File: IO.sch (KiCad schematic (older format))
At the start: 5 parts

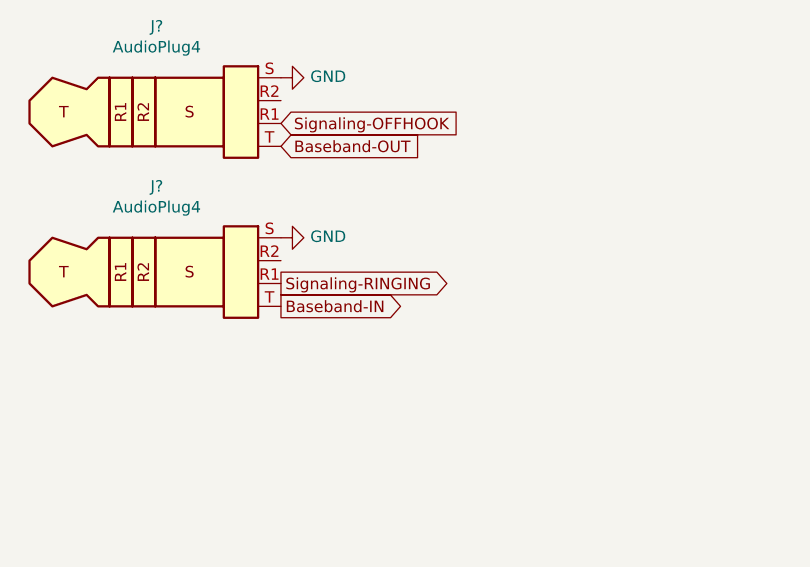
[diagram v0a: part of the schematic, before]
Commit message: more updates
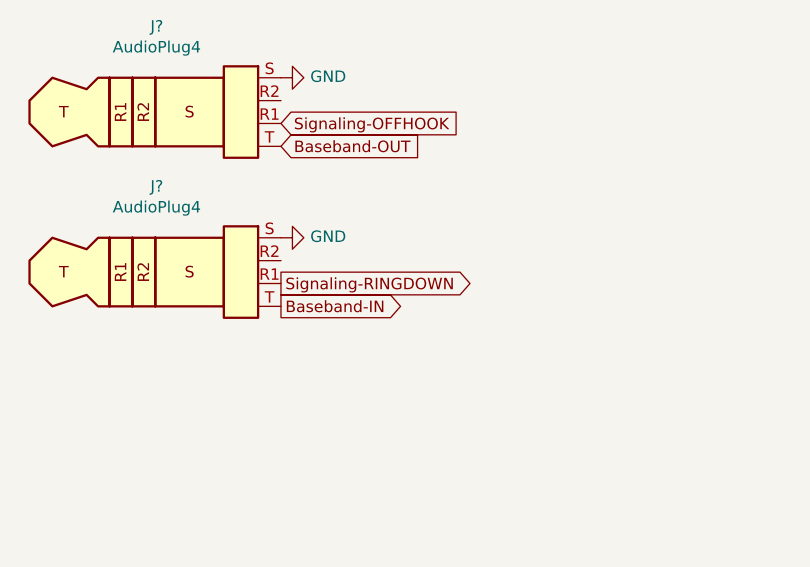
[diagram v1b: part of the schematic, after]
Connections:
- net Signaling-RINGING: no longer J?.R1
- new net Signaling-RINGDOWN: J?.R1
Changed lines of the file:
@@
 Baseband-IN
 Text GLabel 2450 2150 2    50   Output ~ 0
-Signaling-RINGING
+Signaling-RINGDOWN
 Text Notes 850  1050 0    50   ~ 0
 Audio Jack

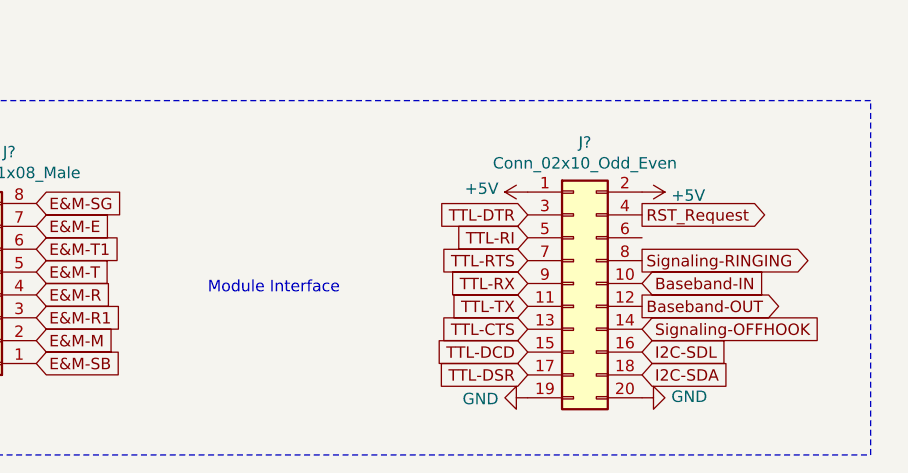
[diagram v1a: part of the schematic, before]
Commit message: updates
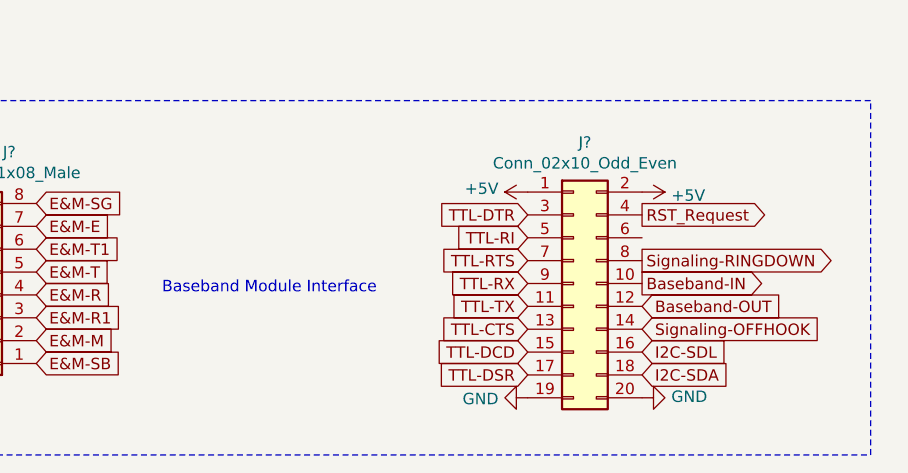
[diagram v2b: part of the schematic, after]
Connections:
- net Signaling-RINGING is gone; now on net Signaling-RINGDOWN: J?.8 (Pin_8)
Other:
- note added: "Baseband Module Interface"
- note removed: "Module Interface"
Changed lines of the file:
@@
 $Descr A4 11693 8268
 encoding utf-8
-Sheet 6 10
+Sheet 6 11
 Title "300 Baud Audio FSK Modem "
 Date "2021-07-08"
@@
 	0    -1   -1   0
 $EndComp
-Text GLabel 7100 4450 2    50   Input ~ 0
+Text GLabel 7100 4450 2    50   Output ~ 0
 Baseband-IN
-Text GLabel 7100 4550 2    50   Output ~ 0
+Text GLabel 7100 4550 2    50   Input ~ 0
 Baseband-OUT
 Text GLabel 7100 4650 2    50   Input ~ 0
@@
 E&M-SG
 Text GLabel 7100 4350 2    50   Output ~ 0
-Signaling-RINGING
+Signaling-RINGDOWN
 $Comp
 L power:GND #PWR?
@@
 	1    0    0    -1
 $EndComp
-Text Notes 5200 4500 0    50   ~ 0
-Module Interface
+Text Notes 5000 4500 0    50   ~ 0
+Baseband Module Interface
 Text GLabel 2350 4450 2    50   Input ~ 0
 E&M-R

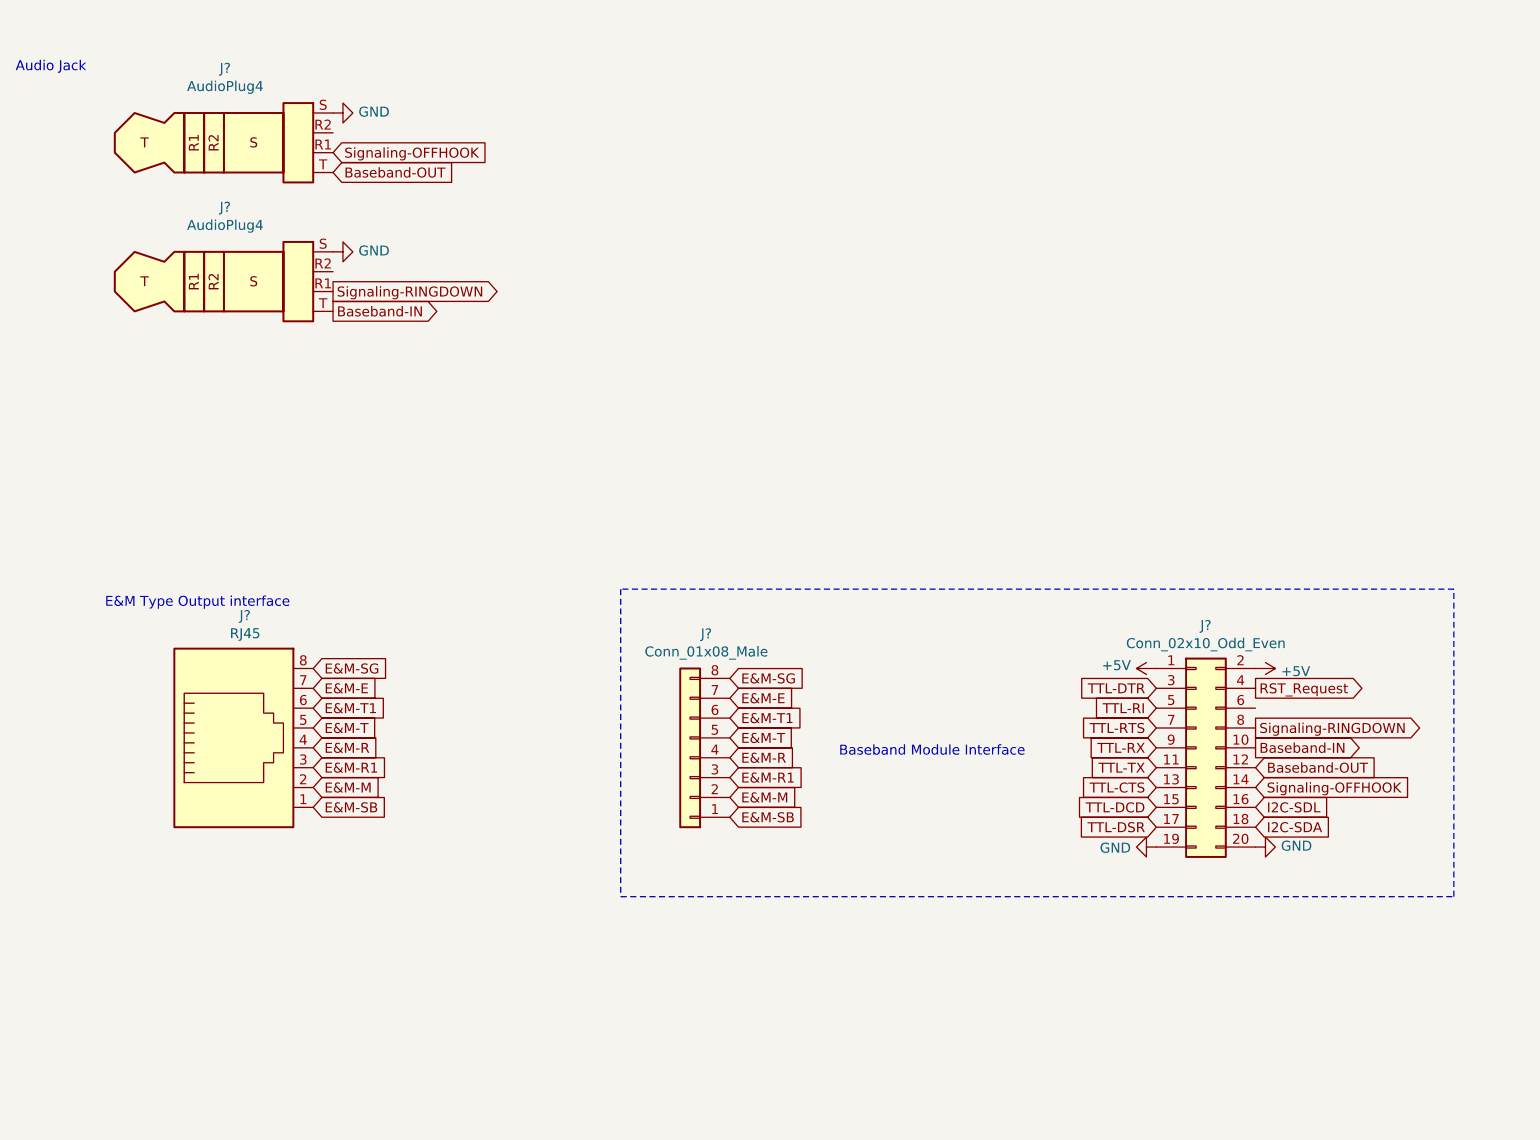
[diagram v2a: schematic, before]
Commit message: updates
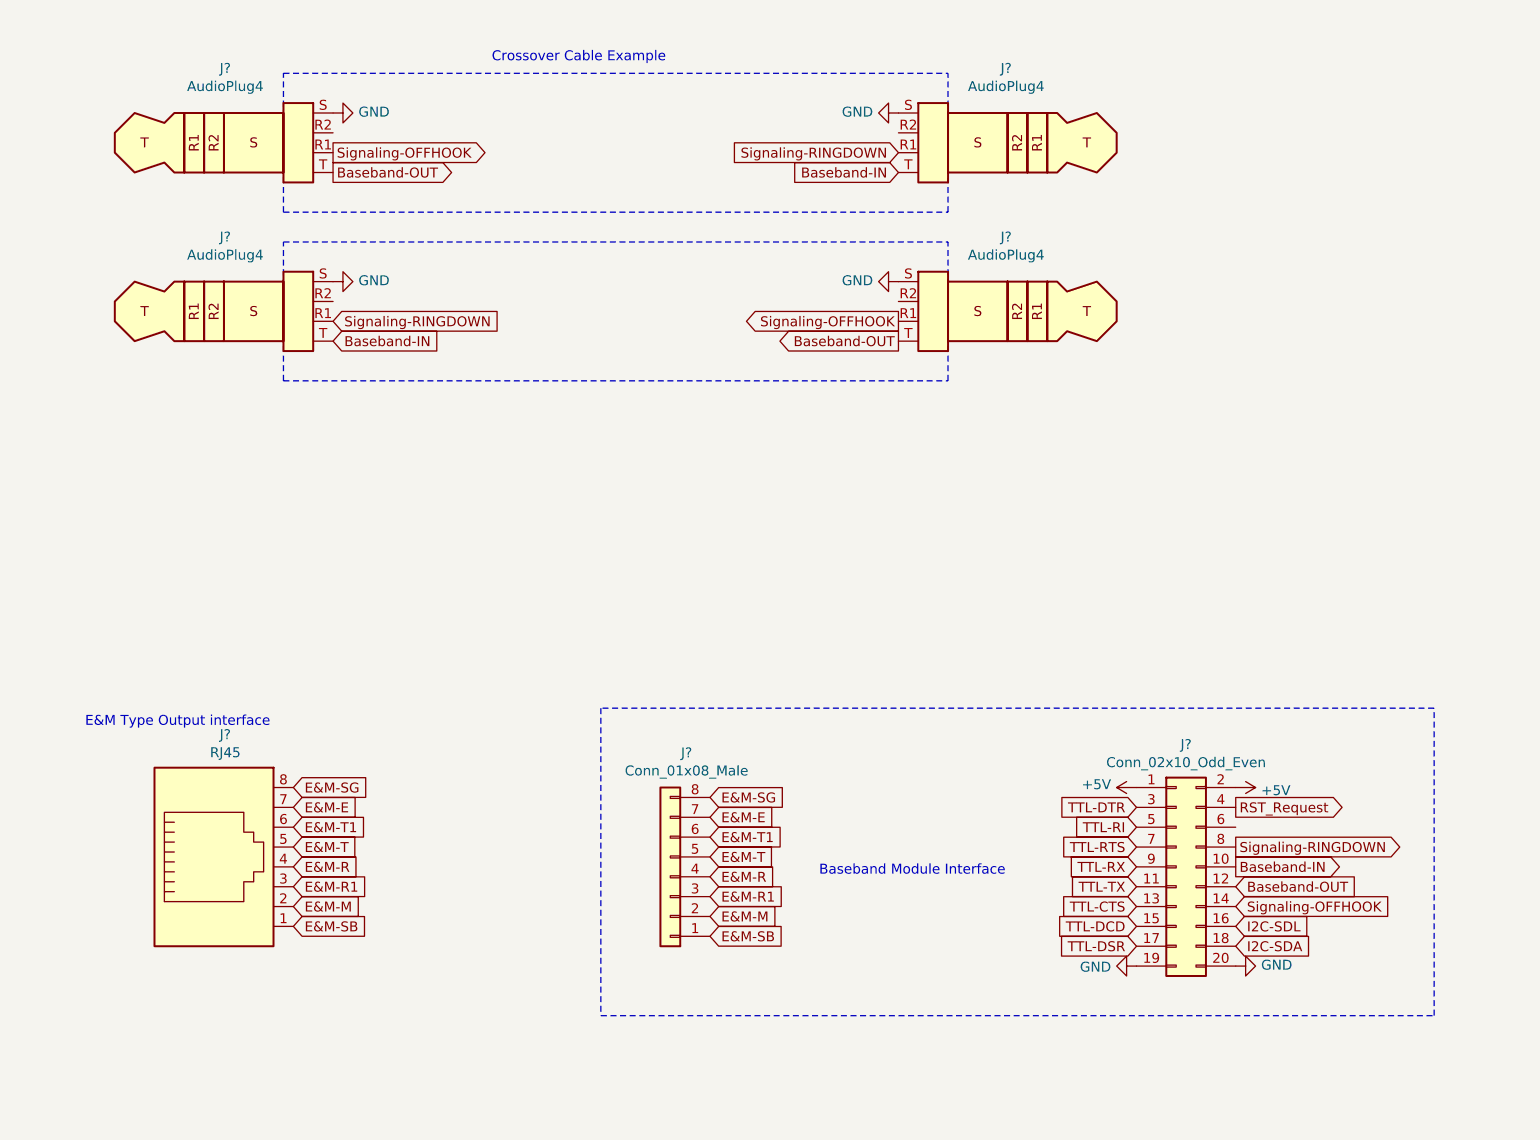
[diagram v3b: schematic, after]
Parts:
- added J? (x2): AudioPlug4, symbol Connector:AudioPlug4
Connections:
- net Baseband-IN: now also J?.T
- net Baseband-OUT: now also J?.T
- net GND: now also J?.S, J?.S
- net Signaling-OFFHOOK: now also J?.R1
- net Signaling-RINGDOWN: now also J?.R1
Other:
- note added: "Crossover Cable Example"
- note removed: "Audio Jack"
- moved on the sheet: J?

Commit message: updates
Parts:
- J? (x2): symbol Connector:AudioPlug4 -> Connector:AudioPlug3
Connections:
- net Baseband-IN: now also J?.R, J?.R; no longer J?.T, J?.T
- net Baseband-OUT: now also J?.T; no longer J?.T
- net GND: now also J?.R2, J?.R2
- net Signaling-OFFHOOK: now also J?.T, J?.T; no longer J?.R1, J?.R1
- net Signaling-RINGDOWN: now also J?.R1; no longer J?.R1
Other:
- note added: "X"
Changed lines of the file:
@@
 RST_Request
 $Comp
-L Connector:AudioPlug4 J?
+L Connector:AudioPlug3 J?
 U 1 1 60EB32CF
-P 1850 1350
+P 1850 1400
 AR Path="/60EB32CF" Ref="J?"  Part="1"
 AR Path="/60E9D9E5/60EB32CF" Ref="J?"  Part="1"
-F 0 "J?" H 1907 1675 50  0000 C CNN
-F 1 "AudioPlug4" H 1907 1584 50  0000 C CNN
-F 2 "" H 2200 1250 50  0001 C CNN
-F 3 "~" H 2200 1250 50  0001 C CNN
-	1    1850 1350
+F 0 "J?" H 1907 1725 50  0000 C CNN
+F 1 "AudioPlug4" H 1907 1634 50  0000 C CNN
+F 2 "" H 2200 1300 50  0001 C CNN
+F 3 "~" H 2200 1300 50  0001 C CNN
+	1    1850 1400
 	1    0    0    -1
 $EndComp
@@
 L power:GND #PWR?
 U 1 1 60EB32D5
-P 2450 1250
+P 2450 1300
 AR Path="/60EB32D5" Ref="#PWR?"  Part="1"
 AR Path="/60E9D9E5/60EB32D5" Ref="#PWR?"  Part="1"
-F 0 "#PWR?" H 2450 1000 50  0001 C CNN
-F 1 "GND" V 2455 1122 50  0000 R CNN
-F 2 "" H 2450 1250 50  0001 C CNN
-F 3 "" H 2450 1250 50  0001 C CNN
-	1    2450 1250
-	0    -1   -1   0
-$EndComp
-Text GLabel 2450 1550 2    50   Output ~ 0
+F 0 "#PWR?" H 2450 1050 50  0001 C CNN
+F 1 "GND" V 2455 1172 50  0000 R CNN
+F 2 "" H 2450 1300 50  0001 C CNN
+F 3 "" H 2450 1300 50  0001 C CNN
+	1    2450 1300
+	0    -1   -1   0
+$EndComp
+Text GLabel 2450 1500 2    50   Output ~ 0
 Baseband-OUT
-Text GLabel 2450 1450 2    50   Output ~ 0
+Text GLabel 2450 2400 2    50   Output ~ 0
 Signaling-OFFHOOK
 Wire Notes Line
@@
 	8000 4250 3800 4250
 $Comp
-L Connector:AudioPlug4 J?
+L Connector:AudioPlug3 J?
 U 1 1 60EE43AB
-P 5900 1350
+P 5900 1400
 AR Path="/60EE43AB" Ref="J?"  Part="1"
 AR Path="/60E9D9E5/60EE43AB" Ref="J?"  Part="1"
-F 0 "J?" H 5957 1675 50  0000 C CNN
-F 1 "AudioPlug4" H 5957 1584 50  0000 C CNN
-F 2 "" H 6250 1250 50  0001 C CNN
-F 3 "~" H 6250 1250 50  0001 C CNN
-	1    5900 1350
+F 0 "J?" H 5957 1725 50  0000 C CNN
+F 1 "AudioPlug4" H 5957 1634 50  0000 C CNN
+F 2 "" H 6250 1300 50  0001 C CNN
+F 3 "~" H 6250 1300 50  0001 C CNN
+	1    5900 1400
 	-1   0    0    -1
 $EndComp
@@
 L power:GND #PWR?
 U 1 1 60EE44F5
-P 5300 1250
+P 5300 1300
 AR Path="/60EE44F5" Ref="#PWR?"  Part="1"
 AR Path="/60E9D9E5/60EE44F5" Ref="#PWR?"  Part="1"
-F 0 "#PWR?" H 5300 1000 50  0001 C CNN
-F 1 "GND" V 5305 1122 50  0000 R CNN
-F 2 "" H 5300 1250 50  0001 C CNN
-F 3 "" H 5300 1250 50  0001 C CNN
-	1    5300 1250
+F 0 "#PWR?" H 5300 1050 50  0001 C CNN
+F 1 "GND" V 5305 1172 50  0000 R CNN
+F 2 "" H 5300 1300 50  0001 C CNN
+F 3 "" H 5300 1300 50  0001 C CNN
+	1    5300 1300
 	0    1    -1   0
 $EndComp
-Text GLabel 5300 1550 0    50   Input ~ 0
+Text GLabel 5300 1400 0    50   Input ~ 0
 Baseband-IN
-Text GLabel 5300 1450 0    50   Input ~ 0
+Text GLabel 5300 2300 0    50   Input ~ 0
 Signaling-RINGDOWN
 Text Notes 3250 1000 0    50   ~ 0
@@
 	0    -1   -1   0
 $EndComp
+Text GLabel 5300 1500 0    50   Output ~ 0
+Baseband-OUT
 Text GLabel 5300 2400 0    50   Output ~ 0
-Baseband-OUT
-Text GLabel 5300 2300 0    50   Output ~ 0
 Signaling-OFFHOOK
 $Comp
@@
 	0    1    -1   0
 $EndComp
-Text GLabel 2450 2400 2    50   Input ~ 0
+Text GLabel 2450 1400 2    50   Input ~ 0
 Baseband-IN
 Text GLabel 2450 2300 2    50   Input ~ 0
@@
 Wire Notes Line
 	2200 2600 2200 1900
+Text Notes 3800 1450 0    50   ~ 0
+X
+$Comp
+L power:GND #PWR?
+U 1 1 60ECC43D
+P 2450 2200
+AR Path="/60ECC43D" Ref="#PWR?"  Part="1"
+AR Path="/60E9D9E5/60ECC43D" Ref="#PWR?"  Part="1"
+F 0 "#PWR?" H 2450 1950 50  0001 C CNN
+F 1 "GND" V 2455 2072 50  0000 R CNN
+F 2 "" H 2450 2200 50  0001 C CNN
+F 3 "" H 2450 2200 50  0001 C CNN
+	1    2450 2200
+	0    -1   -1   0
+$EndComp
+$Comp
+L power:GND #PWR?
+U 1 1 60ECC77D
+P 5300 2200
+AR Path="/60ECC77D" Ref="#PWR?"  Part="1"
+AR Path="/60E9D9E5/60ECC77D" Ref="#PWR?"  Part="1"
+F 0 "#PWR?" H 5300 1950 50  0001 C CNN
+F 1 "GND" V 5305 2072 50  0000 R CNN
+F 2 "" H 5300 2200 50  0001 C CNN
+F 3 "" H 5300 2200 50  0001 C CNN
+	1    5300 2200
+	0    1    -1   0
+$EndComp
+Text Notes 3800 2400 0    50   ~ 0
+X
 $EndSCHEMATC
